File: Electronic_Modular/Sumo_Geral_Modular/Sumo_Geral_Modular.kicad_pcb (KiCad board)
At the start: 2 copper layers, 43 parts, among them J1 Bateria, J10 ESC1, J11 ESC2, J12 USB_B_Micro, J13 SENSOR DE MOUSE, J14 ALIMENTAÇÃO SDM, J15 MPU, J2 VL53L0X 1, J3 VL53L0X 2, J4 VL53L0X 3, J5 VS1838B, J6 ponte H ld e, J7 ponte H ld d, J8 Conn_01x02, J9 Conn_01x02, Q1 S8050, Q2 S8050, SW1 SW_Push, SW2 SW_Push, SW3 SW_Push, U1 AMS1117-5.0, U2 AMS1117-3.3, U3 CH340C, U4 ESP32-WROOM-32UE

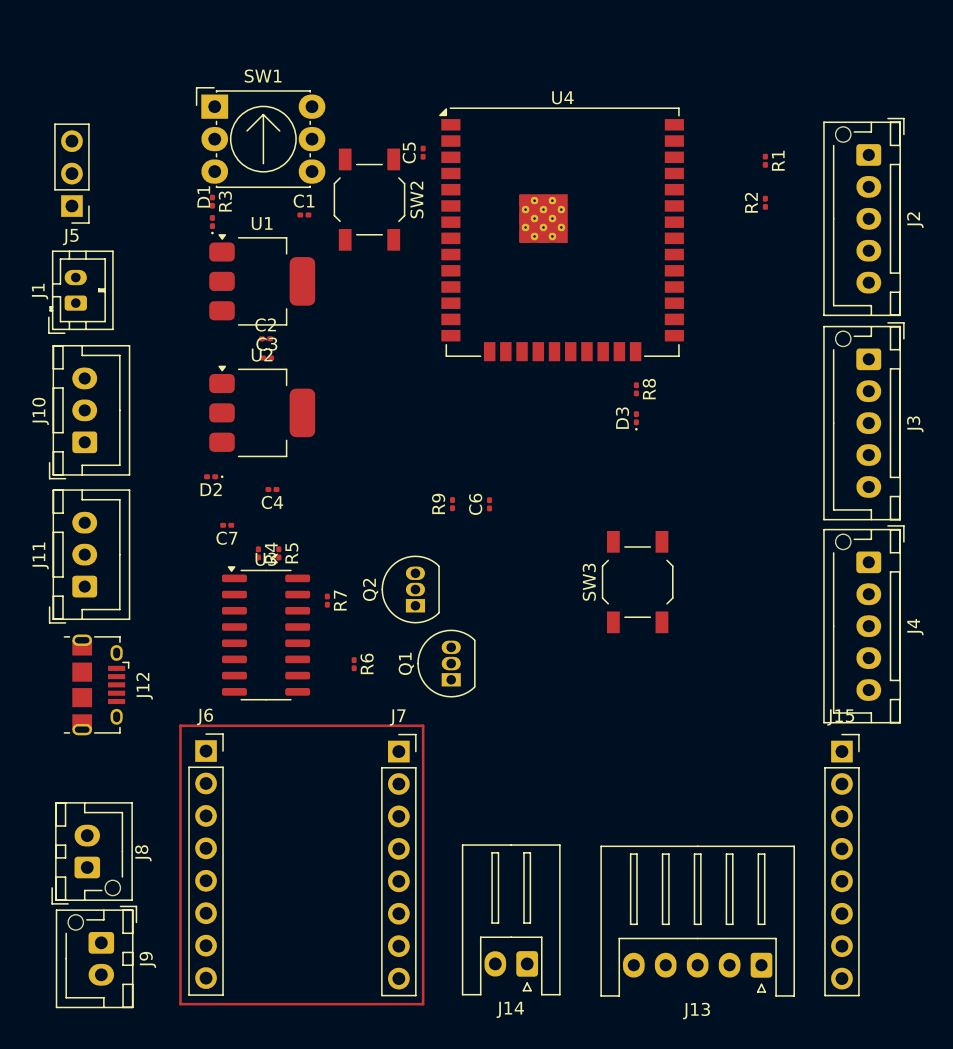
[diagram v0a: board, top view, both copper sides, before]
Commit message: shore: PCB review
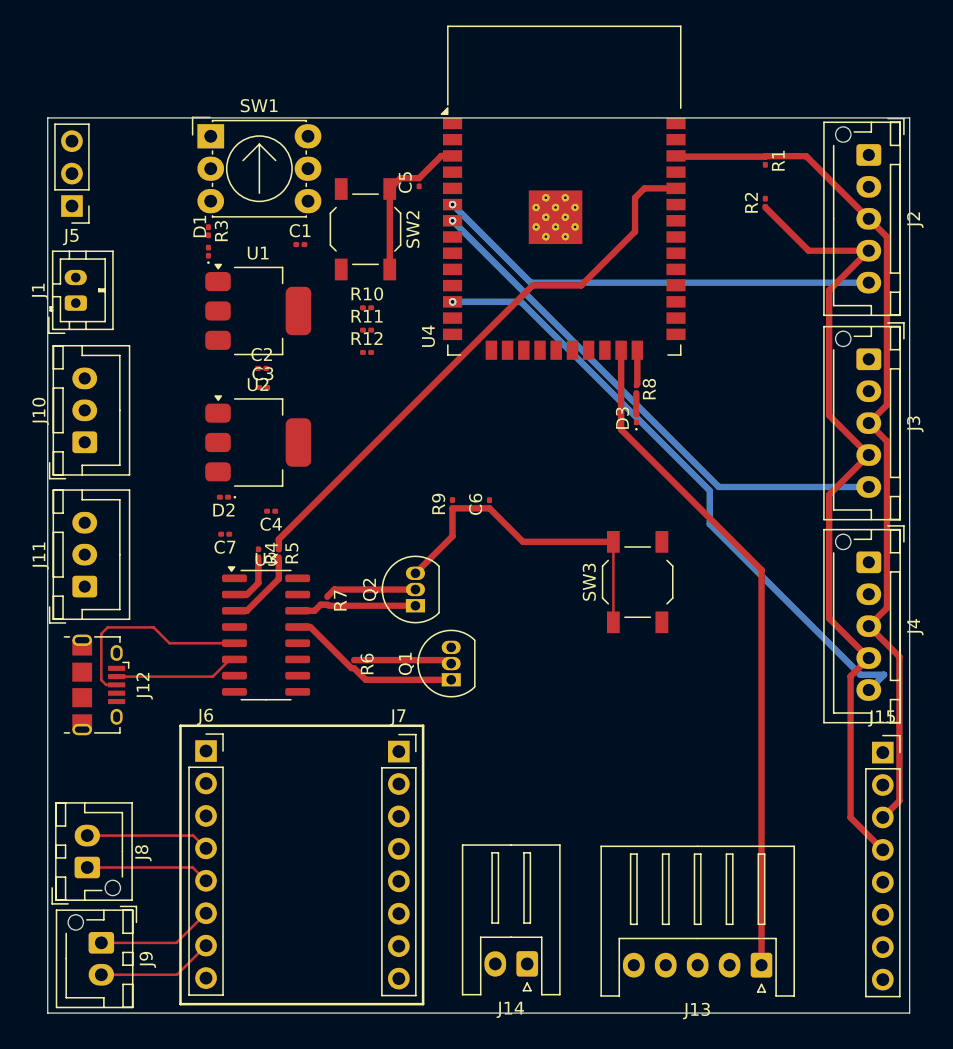
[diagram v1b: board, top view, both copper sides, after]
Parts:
- added R10: 10K, Resistor_SMD:R_0201_0603Metric, F.Cu at (106.6, 39.8)
- added R11: 10K, Resistor_SMD:R_0201_0603Metric, F.Cu at (106.6, 41.5)
- added R12: 10K, Resistor_SMD:R_0201_0603Metric, F.Cu at (106.6, 43.3)
- U4: footprint RF_Module:ESP32-WROOM-32UE -> RF_Module:ESP32-WROOM-32
- moved J15 3.20 mm to (147.0, 74.6)
- moved C1 2.34 mm to (101.4, 34.8)
- moved D1 2.34 mm to (94.2, 35.4)
- moved R3 2.34 mm to (94.2, 33.8)
- moved U2 2.34 mm to (98.1, 50.3)
- moved C5 2.34 mm to (110.7, 29.9)
- moved SW1 2.34 mm to (94.4, 26.3)
- moved SW2 2.34 mm to (106.5, 33.6)
- moved C2 2.34 mm to (98.4, 44.5)
- moved C3 2.34 mm to (98.5, 46.0)
- moved U1 2.34 mm to (98.1, 40.0)
- moved D2 1.89 mm to (95.4, 54.6)
- moved C4 1.70 mm to (99.1, 55.7)
- moved C7 0.72 mm to (95.5, 57.5)
- moved U4 0.30 mm to (122.1, 33.6)
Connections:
- U4 pad 16: unconnected-(U4-IO13-Pad16) -> INT
- U4 pad 5: unconnected-(U4-SENSOR_VN-Pad5) -> DDT
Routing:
- net SCL: track 0.00 -> 68.0 mm
- net SDA: track 0.00 -> 63.4 mm
- net SS/CS: track 0.00 -> 52.7 mm
- net XSH3: track 0.00 -> 49.1 mm, vias 0 -> 1
- net RXD0: track 0.00 -> 44.8 mm
- net XSH2: track 0.00 -> 41.2 mm, vias 0 -> 1
- net XSH1: track 0.00 -> 35.1 mm, vias 0 -> 1
- net I00: track 0.00 -> 26.4 mm
- net Net-(J12-D+): track 0.00 -> 16.1 mm
- net Net-(Q1-E): track 0.00 -> 13.7 mm
- net EN: track 0.00 -> 12.3 mm
- net Net-(J12-D-): track 0.00 -> 9.78 mm
- net AO2: track 0.00 -> 9.73 mm
- net AO1: track 0.00 -> 9.71 mm
- net Net-(Q2-E): track 0.00 -> 9.46 mm
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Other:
- board outline added: 67.5 x 70.1 mm
